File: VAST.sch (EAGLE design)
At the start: 5 parts, among them U2 MPL3115A2

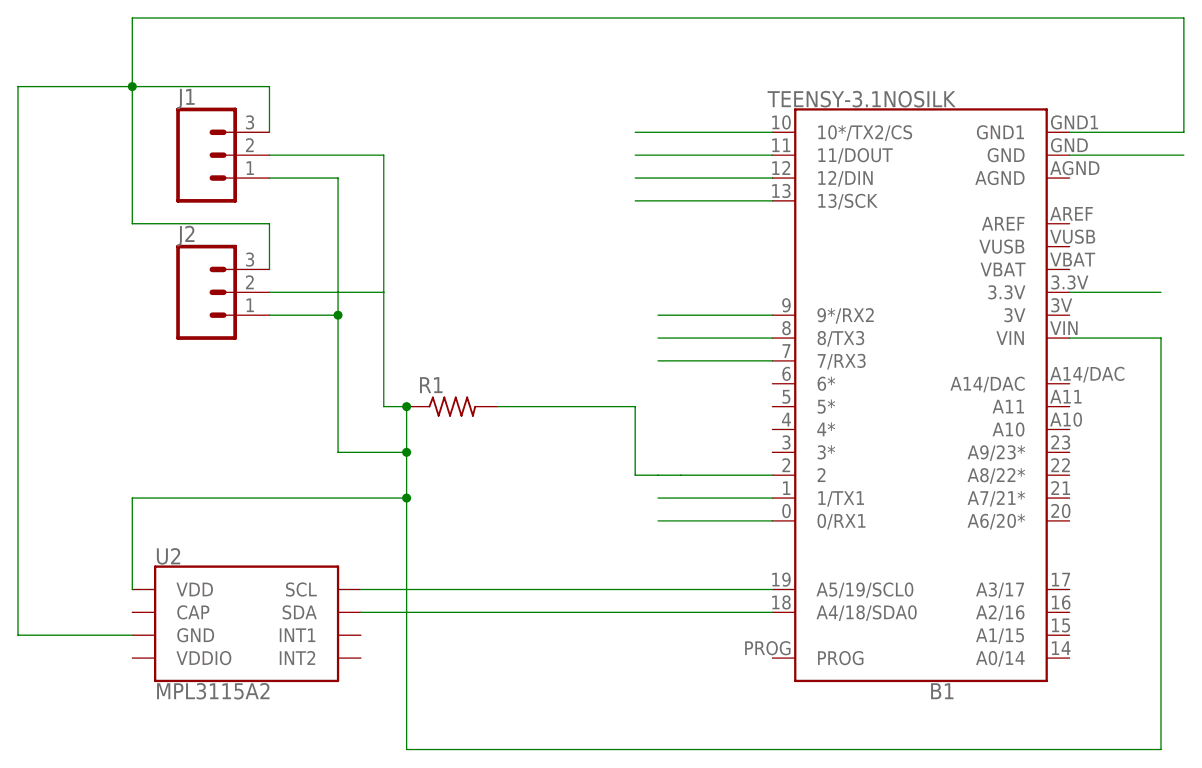
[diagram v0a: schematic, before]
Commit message: Add files via upload
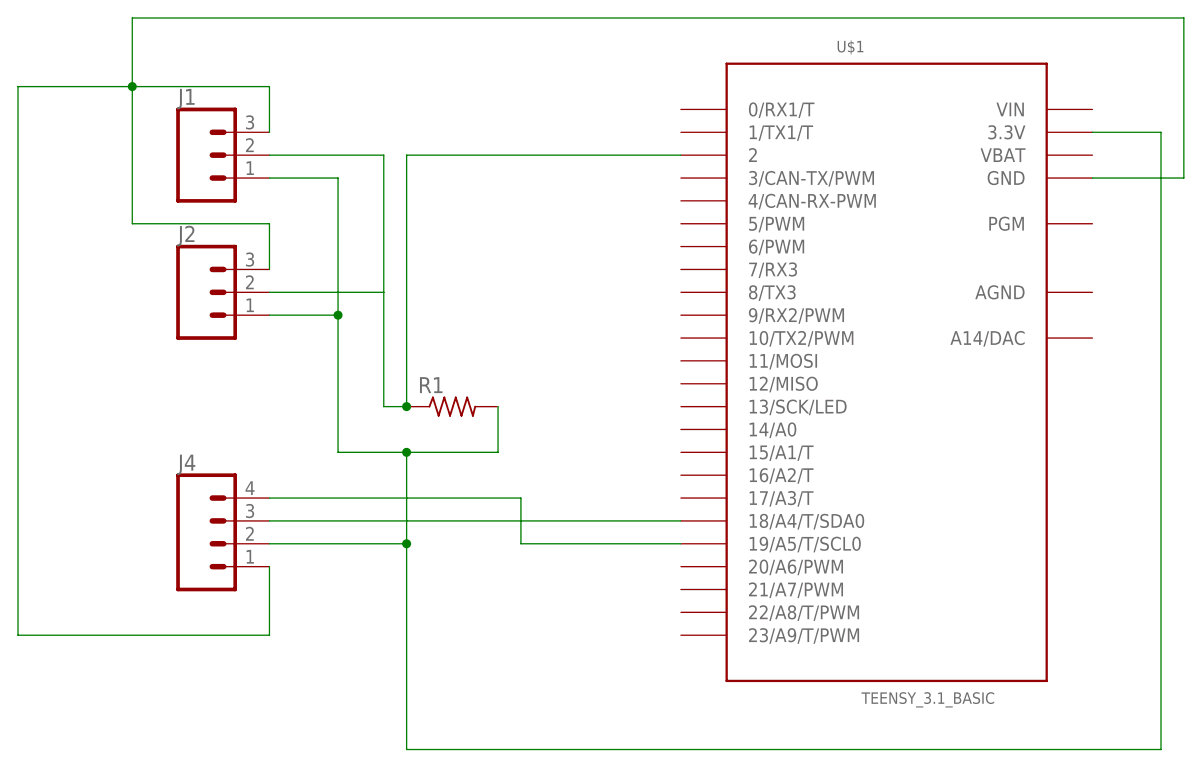
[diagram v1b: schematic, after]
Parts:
- removed B1: TEENSY-3.1NOSILK, SparkFun-Boards:TEENSY-3.1NOSILK
- removed U2: MPL3115A2, SparkFun-Sensors:MPL3115A2
- added J4: (no value), SparkFun-Connectors:CONN_04POLAR
- added U$1: TEENSY_3.1_BASIC, Teensy_3_Series_Board_v1.0:TEENSY_3.1_BASIC
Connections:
- removed net N$10: B1.7/RX3
- removed net N$11: B1.8/TX3
- removed net N$12: B1.9*/RX2
- removed net N$14: B1.GND
- removed net N$16: B1.3.3V
- removed net N$18: B1.VIN, J1.1, J1.2, J2.1, J2.2, R1.1, U2.VDD
- removed net N$5: B1.2, R1.2
- removed net N$6: B1.A4/18/SDA0, U2.SDA
- removed net N$7: B1.A5/19/SCL0, U2.SCL
- removed net N$8: B1.0/RX1
- removed net N$9: B1.1/TX1
- net N$1: now also J1.2, J2.2, R1.1, U$1.2; no longer B1.13/SCK
- net N$13: now also J4.1, U$1.GND; no longer B1.GND1, U2.GND
- net N$2: now also J1.1, J2.1, J4.2, R1.2, U$1.3.3V; no longer B1.12/DIN
- net N$3: now also J4.3, U$1.18/A4/T/SDA0; no longer B1.11/DOUT
- net N$4: now also J4.4, U$1.19/A5/T/SCL0; no longer B1.10*/TX2/CS
